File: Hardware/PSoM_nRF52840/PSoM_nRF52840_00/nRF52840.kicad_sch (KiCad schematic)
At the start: 33 parts, among them J2 U.FL-R-SMT-1_40_, J401 Conn_01x01_Pin, J402 Conn_01x01_Pin, U401 nRF52840-QIAA-aQFN73, Y401 830108161301

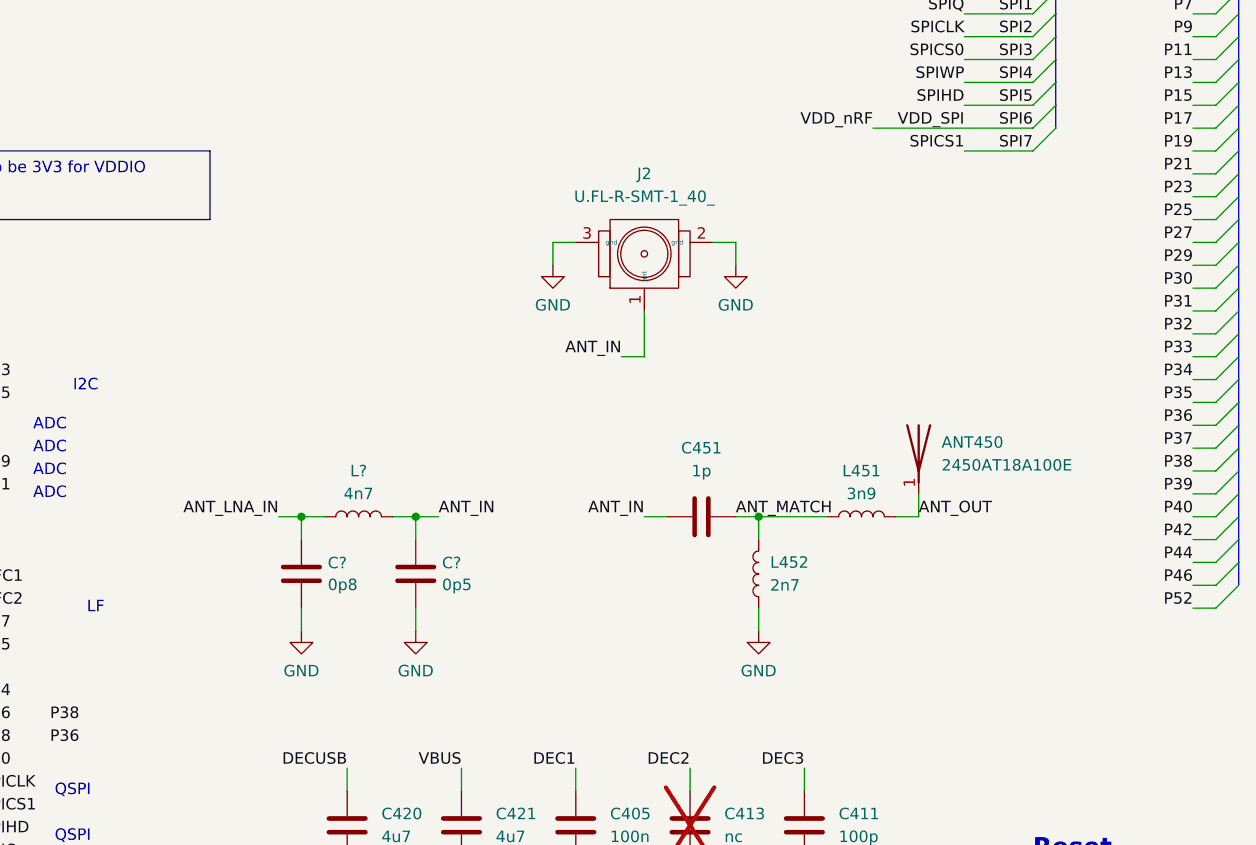
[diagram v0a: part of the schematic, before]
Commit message: finished routing + generated gerbers
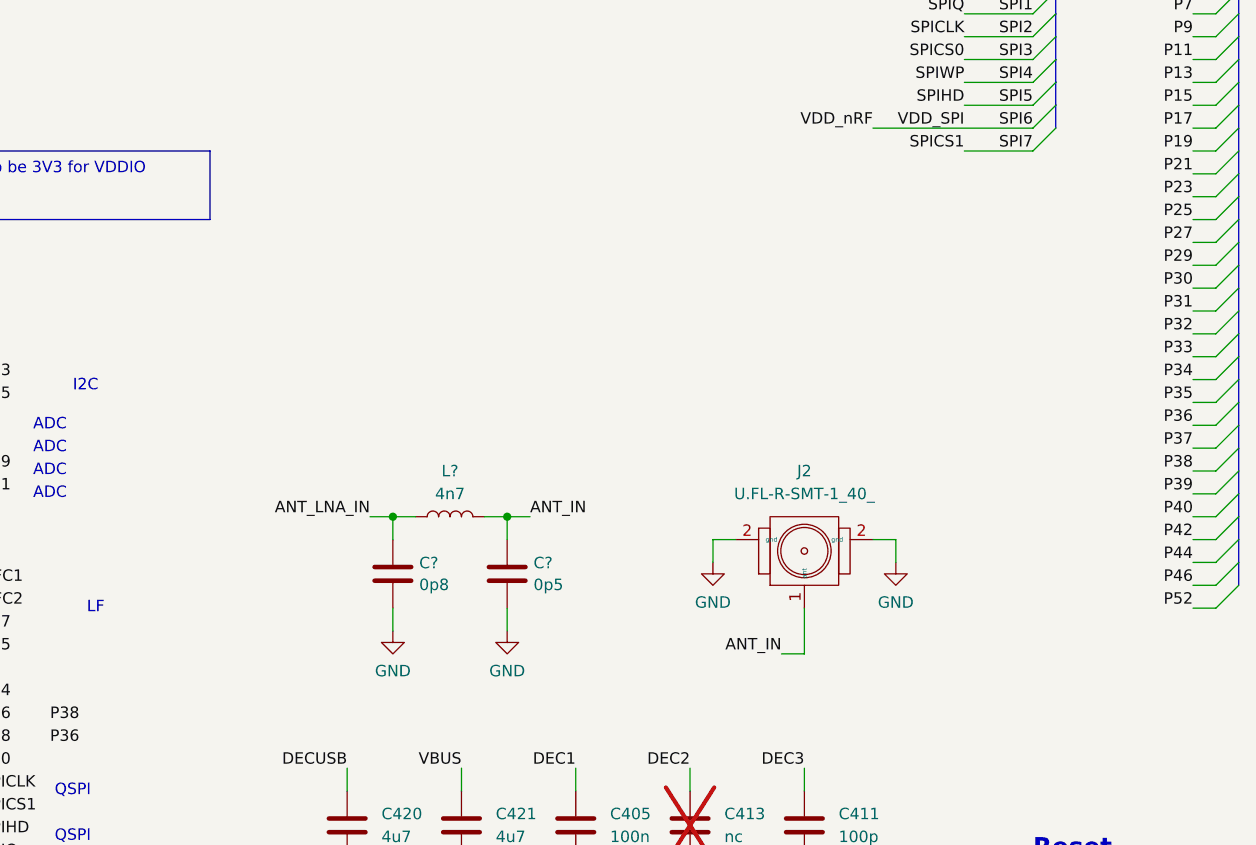
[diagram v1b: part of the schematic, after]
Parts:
- removed ANT450: 2450AT18A100E, Component_lib:ANTC3216X140N, symbol Component_lib:2450AT18A100E
- removed C451: 1p, Capacitor_SMD:C_0201_0603Metric, symbol Component lib:C
- removed L451: 3n9, Inductor_SMD:L_0201_0603Metric, symbol Component lib:L
- removed L452: 2n7, Inductor_SMD:L_0201_0603Metric, symbol Component lib:L
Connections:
- net GND: no longer J2.3 (gnd)
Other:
- moved on the sheet: C?, J2, L?
